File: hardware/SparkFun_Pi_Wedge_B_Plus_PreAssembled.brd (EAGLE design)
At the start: 82.5 x 67.3 mm, 15 parts

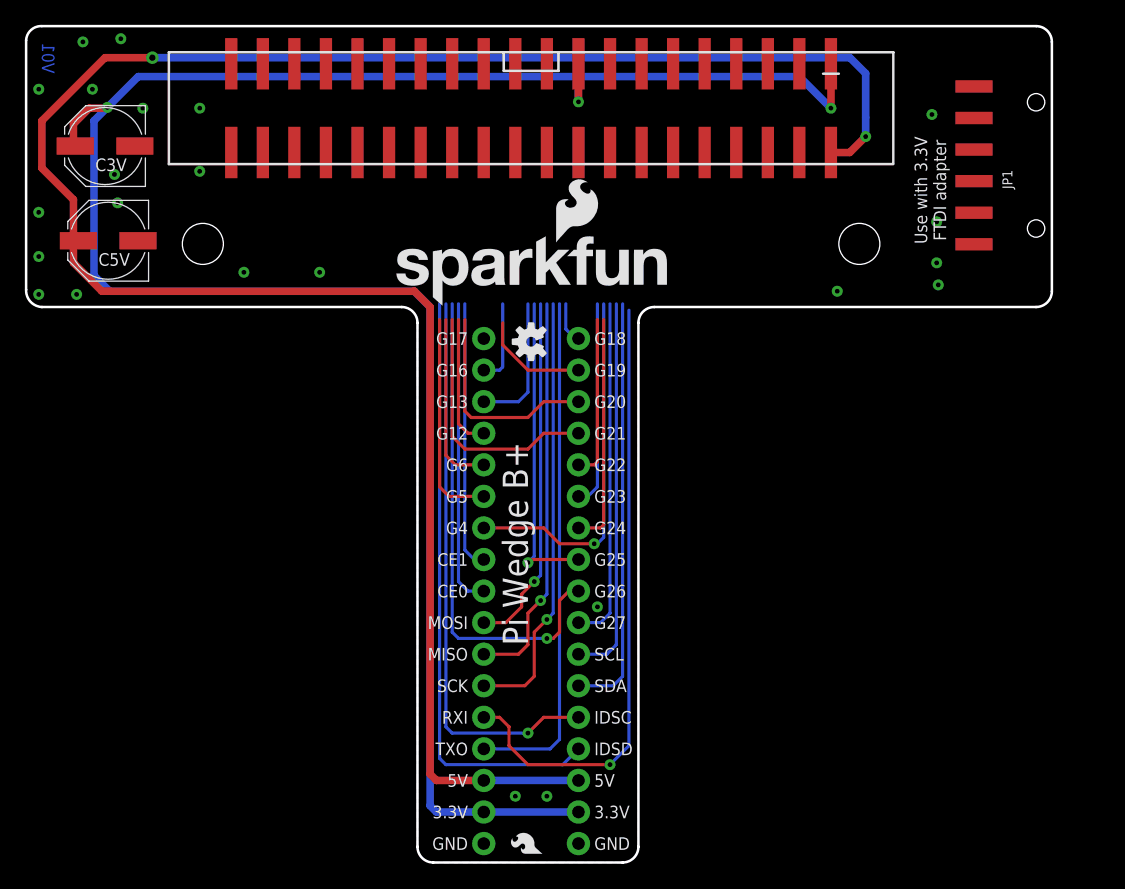
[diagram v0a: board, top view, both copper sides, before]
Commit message: The hard part is routed.
Ready for Review.
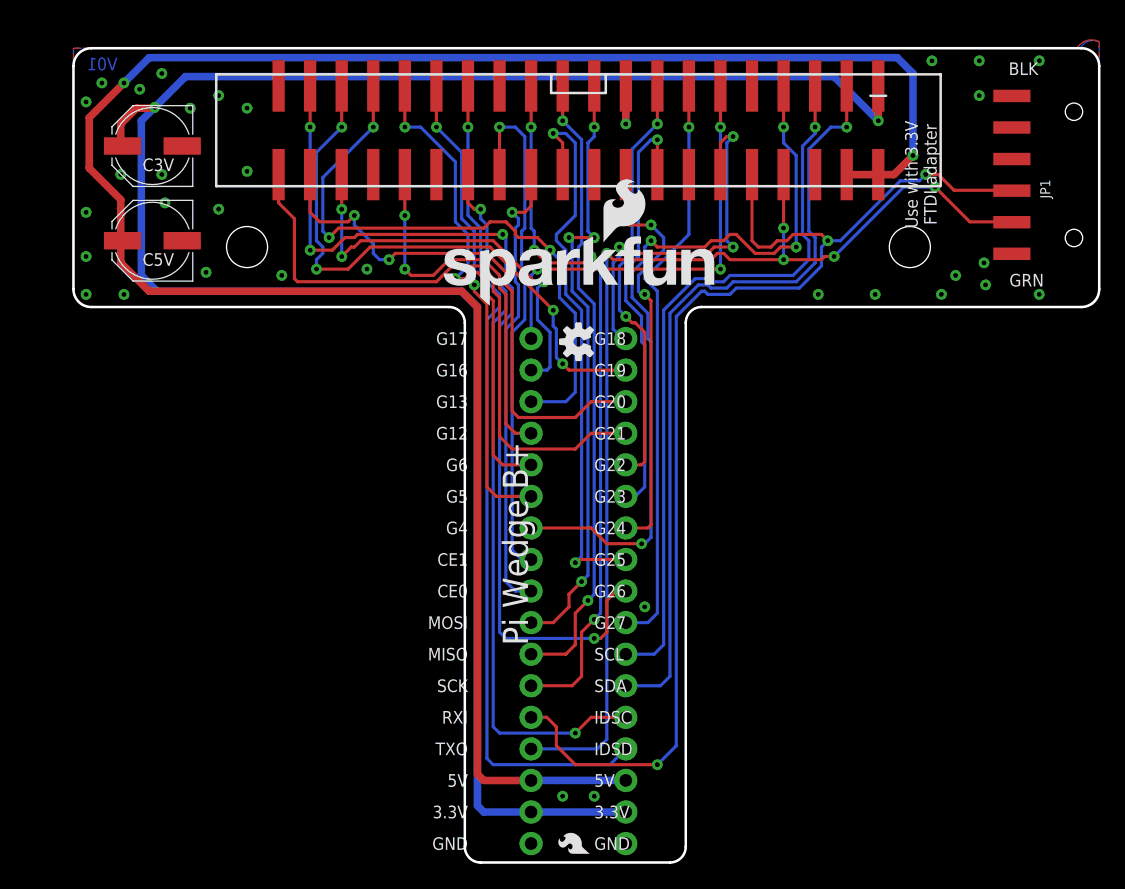
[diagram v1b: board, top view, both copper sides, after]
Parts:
- moved FRAME2 9.43 mm to (19.6, -17.8)
- moved JP2 4.20 mm to (40.6, 58.9)
- moved STANDOFF2 4.07 mm to (67.3, 49.5)
- moved JP4 3.81 mm to (44.5, 1.52)
- moved LOGO2 3.81 mm to (51.8, 44.7)
- moved LOGO4 3.81 mm to (41.8, 2.67)
- moved LOGO5 3.81 mm to (40.6, 41.9)
- moved U$2 3.81 mm to (40.6, 68.8)
- moved C3V 3.81 mm to (6.35, 57.7)
- moved LOGO1 3.81 mm to (29.1, 44.7)
- moved JP3 3.81 mm to (36.8, 1.52)
- moved LOGO3 3.81 mm to (41.9, 0.38)
- moved STANDOFF1 3.57 mm to (14.0, 49.5)
- moved C5V 3.56 mm to (6.35, 50.0)
- moved JP1 3.14 mm to (80.5, 55.3)
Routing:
- net TXO: track 41.5 -> 89.2 mm, vias 0 -> 5
- net RXI: track 49.8 -> 95.0 mm, vias 1 -> 3
- net GP19: track 8.72 -> 47.8 mm, vias 0 -> 4
- net GP13: track 11.0 -> 49.6 mm, vias 0 -> 3
- net GP26: track 39.9 -> 75.4 mm, vias 1 -> 4
- net GP17: track 0.00 -> 35.3 mm, vias 0 -> 3
- net GP4: track 29.2 -> 62.1 mm, vias 1 -> 4
- net GP21: track 20.5 -> 50.0 mm
- net SDA: track 33.8 -> 63.1 mm, vias 0 -> 1
- net SCL: track 30.8 -> 58.5 mm, vias 0 -> 1
- net GP18: track 3.36 -> 30.8 mm, vias 0 -> 3
- net GP16: track 6.71 -> 33.9 mm, vias 0 -> 3
- net GP20: track 17.2 -> 43.8 mm, vias 0 -> 2
- net GP6: track 14.3 -> 39.4 mm, vias 0 -> 2
- net SCLK: track 35.0 -> 57.6 mm, vias 1 -> 4
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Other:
- board size 82.5 x 67.3 mm -> 82.5 x 65.5 mm
- board text added: "2x 0.13" holes Clear 4-40 screws"
- board text added: "All Units In Inches"
- board text added: "BLK"
- board text added: "GRN"
